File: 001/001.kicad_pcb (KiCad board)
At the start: 2 copper layers, 76.2 x 78.7 mm, 7 parts, among them U1 MF-Jalisco, U2 Firma, U3 PinBase, U4 FirmaMH_Jalisco

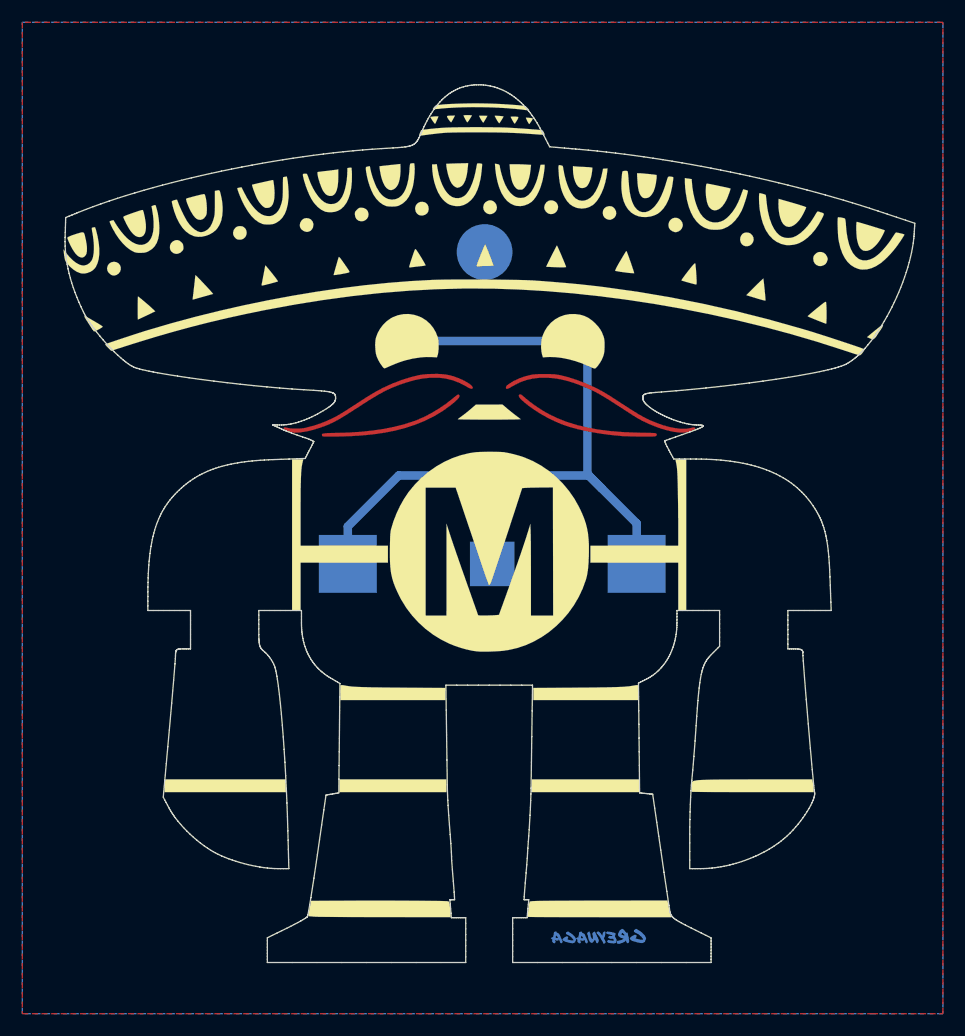
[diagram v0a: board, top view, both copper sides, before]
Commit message: update
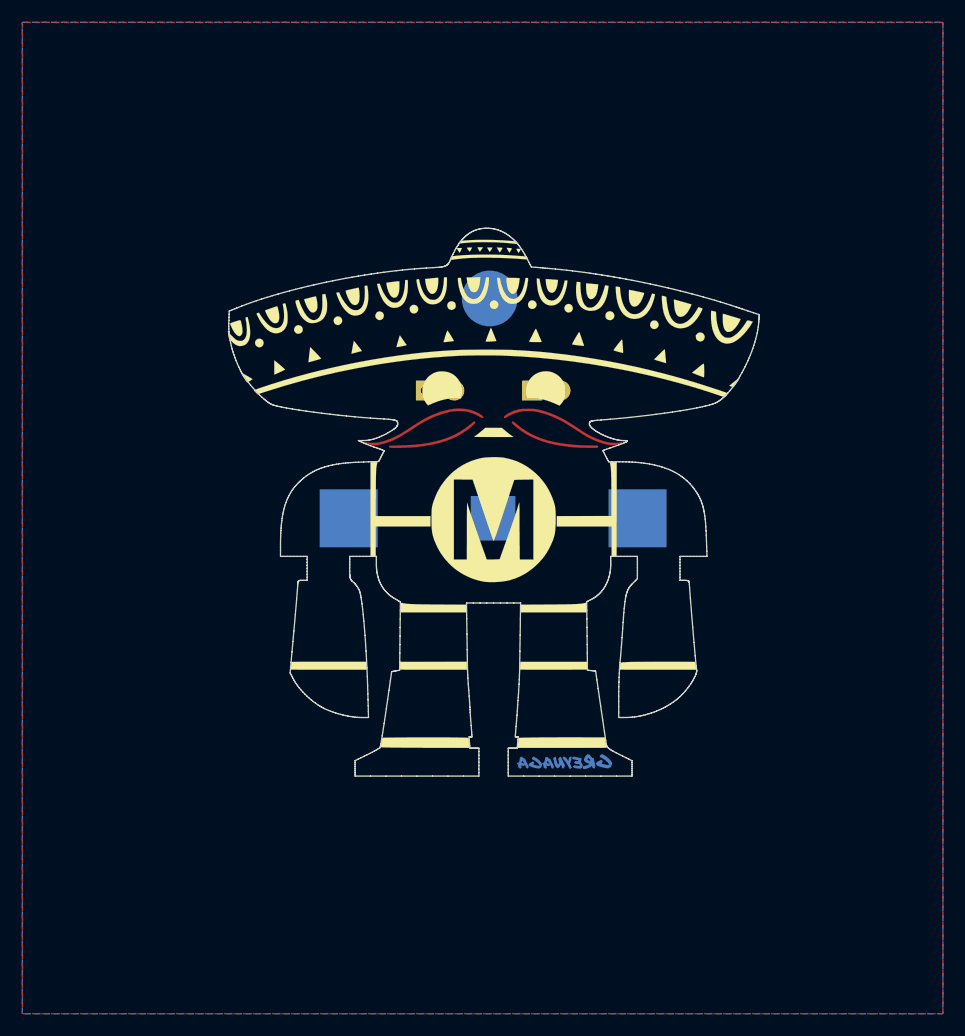
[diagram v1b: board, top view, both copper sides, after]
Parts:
- removed U4: FirmaMH_Jalisco, MF-Jalisco:001_firma_MF
- BT1: footprint 001:WA-BCMC -> MF-Jalisco:WA-BCMC
- U1: footprint MF-Jalisco:MF-Jalisco-001 -> MF-Jalisco:MF-Jalisco_50mm
- moved U2 16.0 mm to (143.9, 123.4)
- moved D1 5.36 mm to (131.4, 90.2)
- moved D2 5.06 mm to (141.0, 90.2)
- moved U3 4.19 mm to (137.2, 81.9)
- moved BT1 4.09 mm to (137.5, 101.6)
- moved U1 3.25 mm to (137.2, 100.3)
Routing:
- net +3V3: track 50.3 -> 0.00 mm
- net Net-(D1-Pad2): track 12.4 -> 0.00 mm
- net GND: vias 1 -> 0
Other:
- board size 76.2 x 78.7 mm -> 47.6 x 49.1 mm
- board text removed: "+"
- board text removed: "Developed by"
